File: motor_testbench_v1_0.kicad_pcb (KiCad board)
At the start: 4 copper layers, 99.5 x 74.5 mm, 254 parts, among them IC1 PJA3402_R1_00001, IC2 VIA2000SD, IC3 MIE1W0505BGLVH-3R-P, IC4 MCP3564RT-E_ST, J1 Conn_01x05_Pin, J10 Conn_01x02_Pin, J11 Conn_01x02_Pin, J12 Conn_01x02_Pin, J13 Conn_01x04_Pin, J2 Conn_01x01_Pin, J3 Conn_01x01_Pin, J4 Conn_01x22_Pin, J7 V_bat_in, J8 V_bat_out, J9 V_bat_secondary, U10 NCV8114BSN330T1G, U11 TPS7A2055PDBVR, U12 TLV75733PDYDR, U13 TPS7A2050PDBVR, U14 TPS7A2033PDBVR, U15 TPS7A2018PDBVRG4, U16 TPS7A2050PDBVR, U18 TPS7A2033PDBVR, U19 TPS7A2045PDBVR, U3 CZ3A05, U4 OPA2328DR, U5 OPA2328DR, U6 MCP1502T-50E/CHY, U7 TPS62933, U8 TPS62933, U9 OPA2387DR

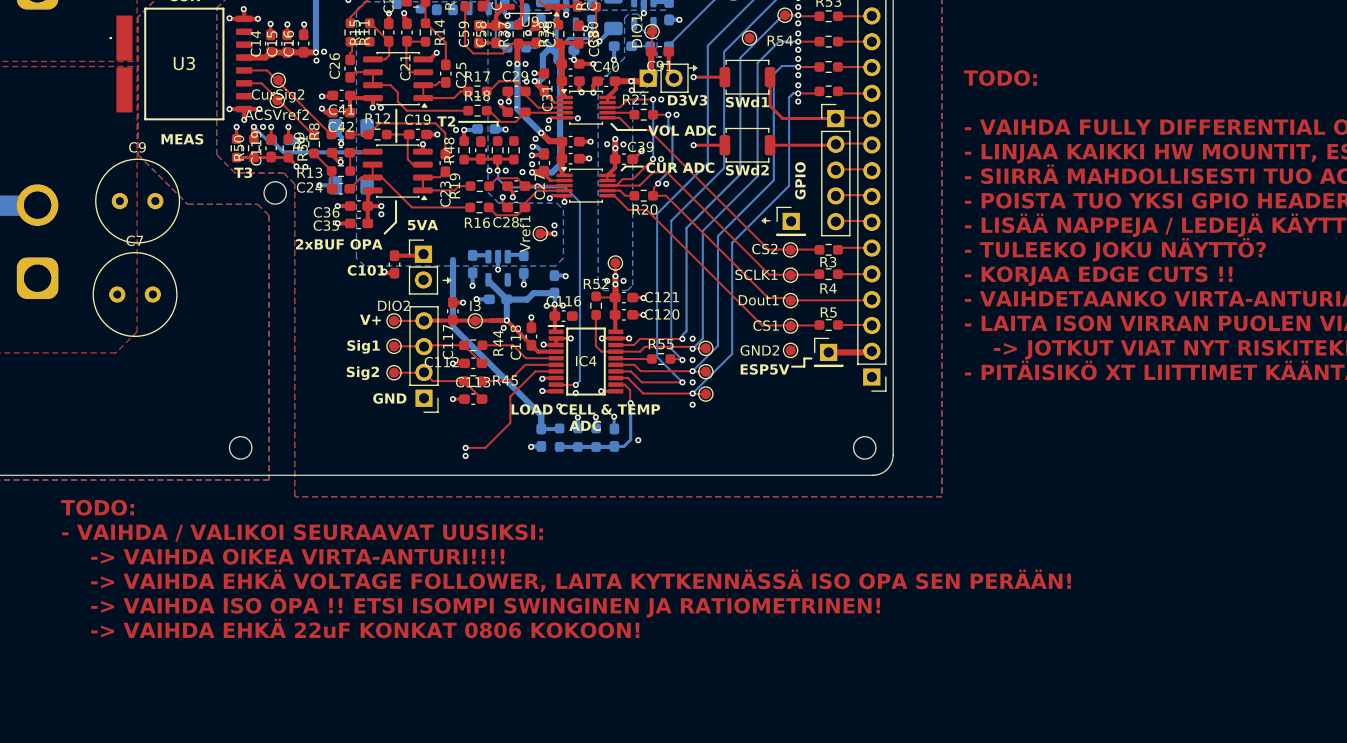
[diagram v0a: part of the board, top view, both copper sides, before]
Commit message: Minor tweaks.
[KiCad Version: 10.0.4]
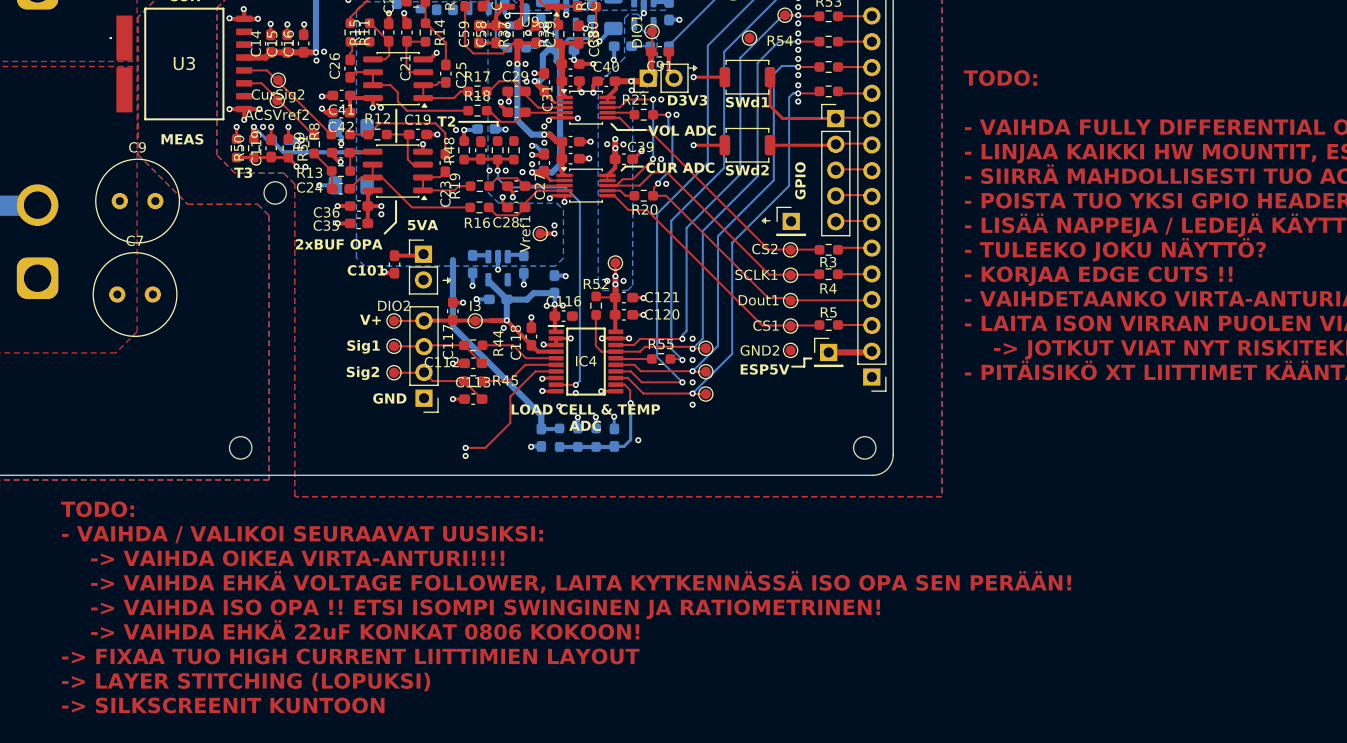
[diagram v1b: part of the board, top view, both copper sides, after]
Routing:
- net +SAR_1_5V_Ref: track 28.2 -> 28.9 mm
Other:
- board text added: "TODO: - VAIHDA / VALIKOI SEURAAVAT UUSIKSI: -> VAIHDA OIKEA VIRTA-ANTURI!!!! -> VAIHDA EHKÄ VOLTAGE FOLLOWER, LAITA KYTKENNÄSSÄ ISO OPA SEN PERÄÄN! -> VAIHDA ISO OPA !! ETSI ISOMPI SWINGINEN JA RATIOMETRINEN! -> VAIHDA EHKÄ 22uF KONKAT 0806 KOKOON! -> FIXAA TUO HIGH CURRENT LIITTIMIEN LAYOUT -> LAYER STITCHING (LOPUKSI) -> SILKSCREENIT KUNTOON"
- board text removed: "TODO: - VAIHDA / VALIKOI SEURAAVAT UUSIKSI: -> VAIHDA OIKEA VIRTA-ANTURI!!!! -> VAIHDA EHKÄ VOLTAGE FOLLOWER, LAITA KYTKENNÄSSÄ ISO OPA SEN PERÄÄN! -> VAIHDA ISO OPA !! ETSI ISOMPI SWINGINEN JA RATIOMETRINEN! -> VAIHDA EHKÄ 22uF KONKAT 0806 KOKOON!"
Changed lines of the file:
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@@
 		(layer "Edge.Cuts")
 	)
-	(gr_text "TODO:\n- VAIHDA / VALIKOI SEURAAVAT UUSIKSI:\n	-> VAIHDA OIKEA VIRTA-ANTURI!!!!\n	-> VAIHDA EHKÄ VOLTAGE FOLLOWER, LAITA KYTKENNÄSSÄ ISO OPA SEN PERÄÄN!\n	-> VAIHDA ISO OPA !! ETSI ISOMPI SWINGINEN JA RATIOMETRINEN!\n	-> VAIHDA EHKÄ 22uF KONKAT 0806 KOKOON!"
-		(at 88.8 130.2 0)
+	(gr_text "TODO:\n- VAIHDA / VALIKOI SEURAAVAT UUSIKSI:\n	-> VAIHDA OIKEA VIRTA-ANTURI!!!!\n	-> VAIHDA EHKÄ VOLTAGE FOLLOWER, LAITA KYTKENNÄSSÄ ISO OPA SEN PERÄÄN!\n	-> VAIHDA ISO OPA !! ETSI ISOMPI SWINGINEN JA RATIOMETRINEN!\n	-> VAIHDA EHKÄ 22uF KONKAT 0806 KOKOON!\n-> FIXAA TUO HIGH CURRENT LIITTIMIEN LAYOUT\n-> LAYER STITCHING (LOPUKSI)\n-> SILKSCREENIT KUNTOON"
+		(at 88.8 137.6 0)
 		(layer "F.Cu")
 		(effects
@@
 	)
 	(segment
-		(start 136.24375 82.475)
-		(end 136.33125 82.3875)
-		(width 0.4)
-		(layer "F.Cu")
-		(net "GND")
-	)
-	(segment
 		(start 115.51 82.46)
 		(end 115.51 82.16)
@@
 	)
 	(segment
-		(start 135.175 82.425)
-		(end 135.225 82.475)
-		(width 0.4)
-		(layer "F.Cu")
-		(net "GND")
-	)
-	(segment
 		(start 151.55 54.71875)
 		(end 151.5 54.76875)
@@
 	)
 	(segment
+		(start 136.24375 82.475)
+		(end 136.33125 82.3875)
+		(width 0.4)
+		(layer "F.Cu")
+		(net "GND")
+	)
+	(segment
 		(start 122.0075 48.14)
 		(end 123.22 48.14)
@@
 	)
 	(segment
+		(start 135.225 82.475)
+		(end 136.24375 82.475)
+		(width 0.4)
+		(layer "F.Cu")
+		(net "GND")
+	)
+	(segment
 		(start 135.431154 74.435213)
 		(end 135.433441 74.4375)
@@
 	)
 	(segment
-		(start 135.225 82.475)
-		(end 136.24375 82.475)
-		(width 0.4)
-		(layer "F.Cu")
-		(net "GND")
-	)
-	(segment
 		(start 137.549 104.425)
 		(end 136.275 104.425)
@@
 	)
 	(segment
-		(start 135.175 82.5)
-		(end 135.175 82.425)
-		(width 0.4)
-		(layer "F.Cu")
-		(net "GND")
-	)
-	(segment
 		(start 128.5375 106.5)
 		(end 127.4 106.5)
@@
 	)
 	(segment
+		(start 135.2 82.45)
+		(end 135.225 82.475)
+		(width 0.4)
+		(layer "F.Cu")
+		(net "GND")
+	)
+	(segment
 		(start 144.32292 43.42375)
 		(end 144.32292 43.62375)
@@
 	)
 	(via
-		(at 135.534313 80.865687)
+		(at 136.4 81.25)
 		(size 0.6)
 		(drill 0.3)
@@
 	)
 	(via
-		(at 135.175 82.5)
+		(at 135.2 82.45)
 		(size 0.6)
 		(drill 0.3)
@@
 	)
 	(via
-		(at 135.25 81.65)
+		(at 135.2 81.55)
 		(size 0.6)
 		(drill 0.3)
@@
 	)
 	(via
-		(at 136.776626 79.845254)
+		(at 136.4 79.65)
 		(size 0.6)
 		(drill 0.3)
@@
 	)
 	(segment
+		(start 135.5625 81.55)
+		(end 136.35 82.3375)
+		(width 0.4)
+		(layer "B.Cu")
+		(net "GND")
+	)
+	(segment
 		(start 134.38125 94.1125)
 		(end 134.38125 95.225)
@@
 	)
 	(segment
-		(start 135.25 81.65)
-		(end 135.6625 81.65)
+		(start 135.175 81.575)
+		(end 135.2 81.55)
 		(width 0.4)
 		(layer "B.Cu")
@@
 	)
 	(segment
-		(start 135.6625 81.65)
-		(end 136.35 82.3375)
-		(width 0.4)
-		(layer "B.Cu")
-		(net "GND")
-	)
-	(segment
 		(start 129.34375 95.3375)
 		(end 129.33125 95.35)
@@
 	)
 	(segment
+		(start 135.2 81.55)
+		(end 135.5625 81.55)
+		(width 0.4)
+		(layer "B.Cu")
+		(net "GND")
+	)
+	(segment
 		(start 136.575 69.625)
 		(end 136.05 69.1)
@@
 	)
 	(segment
+		(start 136.4 80.45)
+		(end 136.95 80.45)
+		(width 0.6)
+		(layer "F.Cu")
+		(net "+SAR_1_5V_Ref")
+	)
+	(segment
 		(start 133.749997 71.575003)
 		(end 133.85 71.475)
@@
 	)
 	(segment
-		(start 136.1 80.3)
-		(end 136.9 81.1)
+		(start 136.95 80.45)
+		(end 137.6 81.1)
 		(width 0.6)
 		(layer "F.Cu")
@@
 	)
 	(segment
-		(start 136.9 81.1)
-		(end 138.075 81.1)
-		(width 0.6)
-		(layer "F.Cu")
-		(net "+SAR_1_5V_Ref")
-	)
-	(segment
 		(start 133.9 71.4625)
 		(end 133.85 71.5125)
@@
 	)
 	(segment
+		(start 138.075 81.1)
+		(end 138.125 81.15)
+		(width 0.6)
+		(layer "F.Cu")
+		(net "+SAR_1_5V_Ref")
+	)
+	(segment
 		(start 129.4 72.4625)
 		(end 132.3375 72.4625)
@@
 	)
 	(segment
+		(start 137.6 81.1)
+		(end 138.075 81.1)
+		(width 0.6)
+		(layer "F.Cu")
+		(net "+SAR_1_5V_Ref")
+	)
+	(segment
 		(start 138.125 82.9184)
 		(end 138.125 83.894)
@@
 	)
 	(segment
-		(start 138.075 81.1)
-		(end 138.125 81.15)
-		(width 0.6)
-		(layer "F.Cu")
-		(net "+SAR_1_5V_Ref")
-	)
-	(segment
 		(start 138.171 82.8724)
 		(end 138.125 82.9184)
@@
 	)
 	(via
-		(at 136.1 80.3)
+		(at 136.4 80.45)
 		(size 0.6)
 		(drill 0.3)
@@
 	)
 	(segment
-		(start 133.749997 73.5)
-		(end 133.749997 77.949997)
+		(start 135.15 80.45)
+		(end 133.749997 79.049997)
+		(width 0.6)
+		(layer "B.Cu")
+		(net "+SAR_1_5V_Ref")
+	)
+	(segment
+		(start 133.749997 79.049997)
+		(end 133.749997 73.5)
+		(width 0.6)
+		(layer "B.Cu")
+		(net "+SAR_1_5V_Ref")
+	)
+	(segment
+		(start 136.068629 80.45)
+		(end 135.15 80.45)
 		(width 0.6)
 		(layer "B.Cu")
@@
 	)
 	(segment
-		(start 133.749997 77.949997)
-		(end 136.1 80.3)
+		(start 136.4 80.45)
+		(end 136.068629 80.45)
 		(width 0.6)
 		(layer "B.Cu")
